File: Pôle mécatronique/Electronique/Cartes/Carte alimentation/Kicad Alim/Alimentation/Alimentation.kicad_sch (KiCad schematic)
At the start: 16 parts, among them J1 Conn_01x04, J2 Conn_01x04, J3 Conn_01x04, J4 Conn_01x05, J5 Conn_01x05, J6 Conn_02x03_Odd_Even, J7 Conn_02x10_Odd_Even, J8 Conn_01x02, J9 Conn_01x02, K1 G5LE-1, Q1 BD135, U1 TSR_2-2450, U2 TSR_2-2450, U3 TSR_2-24120

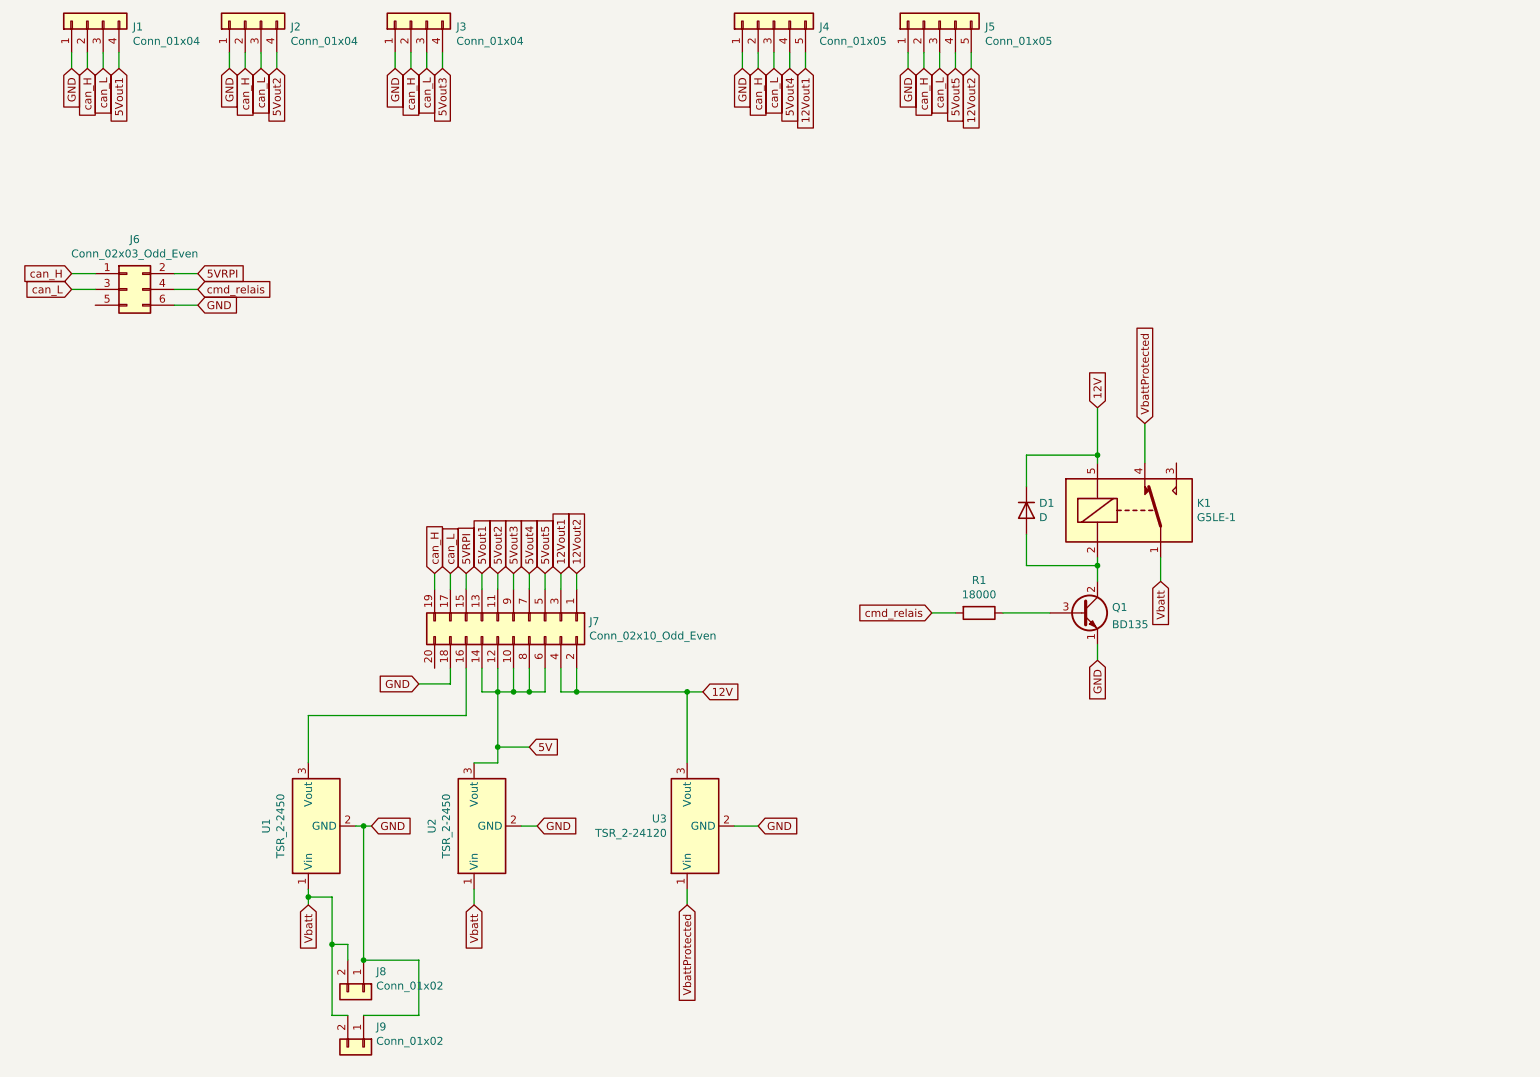
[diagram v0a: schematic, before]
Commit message: Update alim sécurité
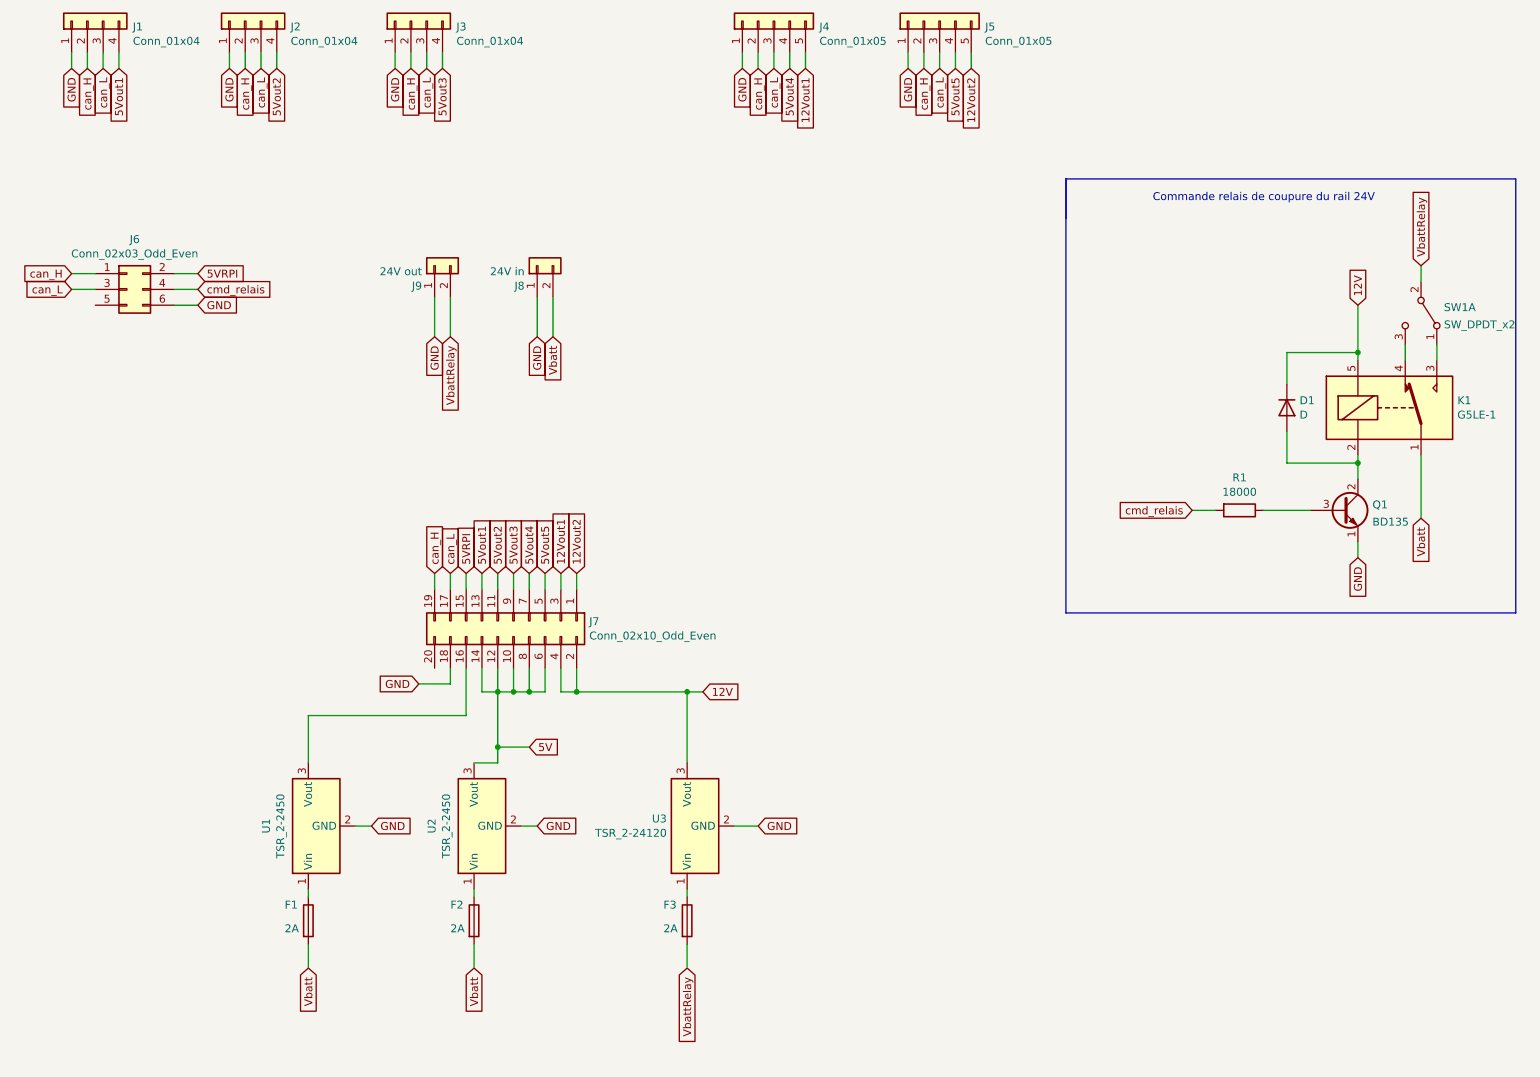
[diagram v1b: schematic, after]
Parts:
- added F1, F2, F3: 2A, Fuse:Fuse_BelFuse_0ZRE0012FF_L8.3mm_W3.8mm, symbol Device:Fuse
- added SW1: SW_DPDT_x2, Autre:Switch_3_Pin, symbol Switch:SW_DPDT_x2
- J8: value Conn_01x02 -> 24V in
- J9: value Conn_01x02 -> 24V out
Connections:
- net Vbatt: now also F1.2, F2.2; no longer J9.2 (Pin_2), U1.1 (Vin), U2.1 (Vin)
- net at K1.3: now also SW1.1 (A)
- net VbattProtected: no longer names the net of U3.1 (Vin)
- net VbattProtected: now also F3.1; no longer K1.4
- new net: F2.1, U2.1 (Vin)
- new net: F1.1, U1.1 (Vin)
- new net: K1.4, SW1.3 (C)
- new net VbattRelay: F3.2, J9.2 (Pin_2), SW1.2 (B)
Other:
- note added: "Commande relais de coupure du rail 24V"
- moved on the sheet: D1, J8, J9, K1, Q1, R1
